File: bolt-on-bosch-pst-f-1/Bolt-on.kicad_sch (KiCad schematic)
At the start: 10 parts

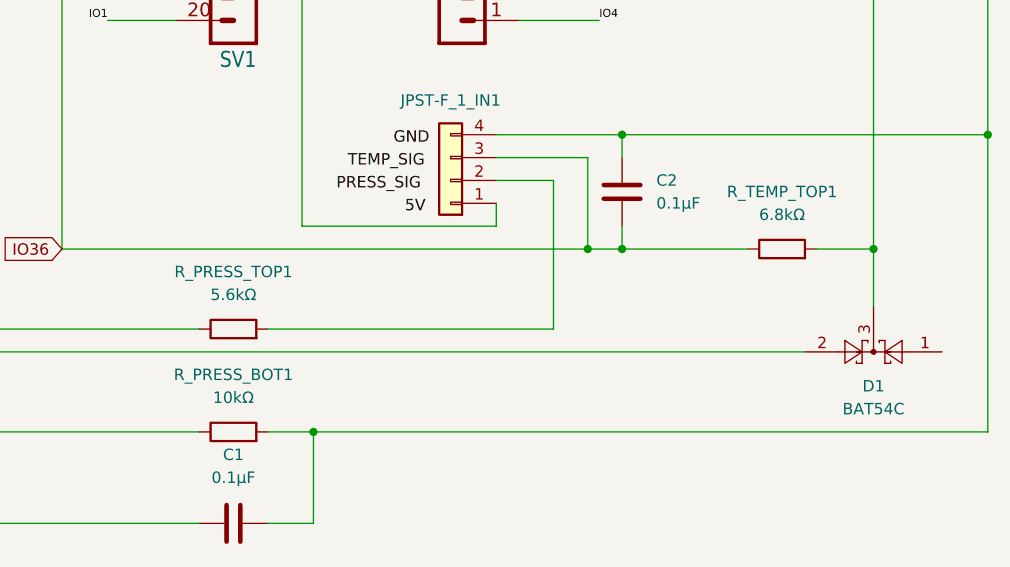
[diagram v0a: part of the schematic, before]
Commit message: cleanup kicad design
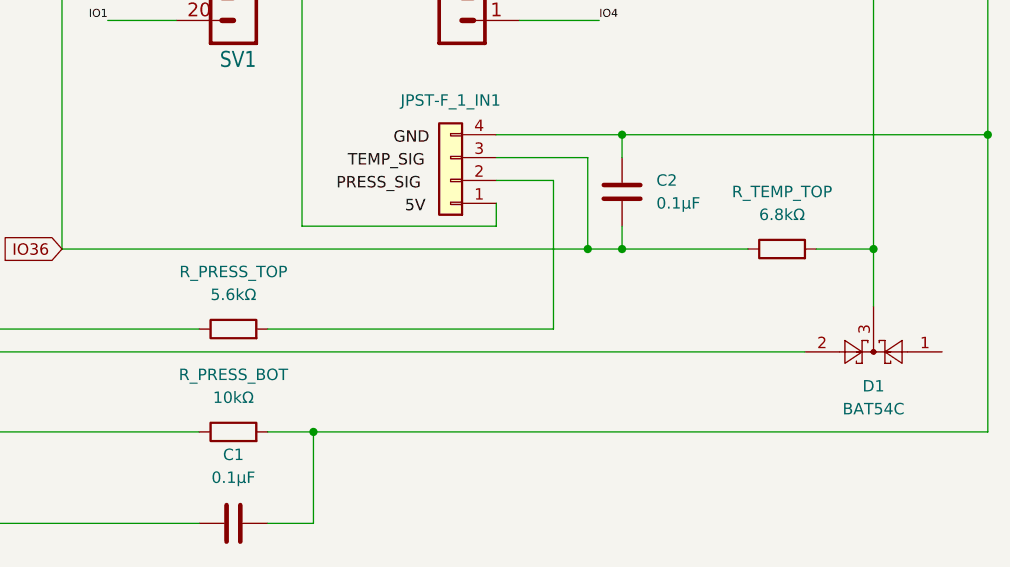
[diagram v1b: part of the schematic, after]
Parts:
- renumbered R_PRESS_BOT1 to R_PRESS_BOT, R_PRESS_TOP1 to R_PRESS_TOP, R_TEMP_TOP1 to R_TEMP_TOP
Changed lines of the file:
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@@
 		(on_board yes)
 		(dnp no)
-		(property "Reference" "R_PRESS_TOP1"
+		(property "Reference" "R_PRESS_TOP"
 			(at 199.39 201.93 90)
 			(effects
@@
 			(project ""
 				(path "/d642a88c-4bf2-433d-8cf9-b5aeaa3805cb"
-					(reference "R_PRESS_TOP1")
+					(reference "R_PRESS_TOP")
 					(unit 1)
 				)
@@
 		(dnp no)
 		(fields_autoplaced yes)
-		(property "Reference" "R_TEMP_TOP1"
+		(property "Reference" "R_TEMP_TOP"
 			(at 260.35 193.04 90)
 			(effects
@@
 			(project "Bolt-on"
 				(path "/d642a88c-4bf2-433d-8cf9-b5aeaa3805cb"
-					(reference "R_TEMP_TOP1")
+					(reference "R_TEMP_TOP")
 					(unit 1)
 				)
@@
 		(dnp no)
 		(fields_autoplaced yes)
-		(property "Reference" "R_PRESS_BOT1"
+		(property "Reference" "R_PRESS_BOT"
 			(at 199.39 213.36 90)
 			(effects
@@
 			(project "Bolt-on"
 				(path "/d642a88c-4bf2-433d-8cf9-b5aeaa3805cb"
-					(reference "R_PRESS_BOT1")
-					(unit 1)
-				)
+					(reference "R_PRESS_BOT")
+					(unit 1)
+				)
